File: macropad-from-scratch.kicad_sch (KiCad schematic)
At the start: 23 parts, among them J1 AVR-ISP-6, U1 PRTR5V0U2X, U2 ATmega32U4-A, Y1 Crystal_GND24_Small

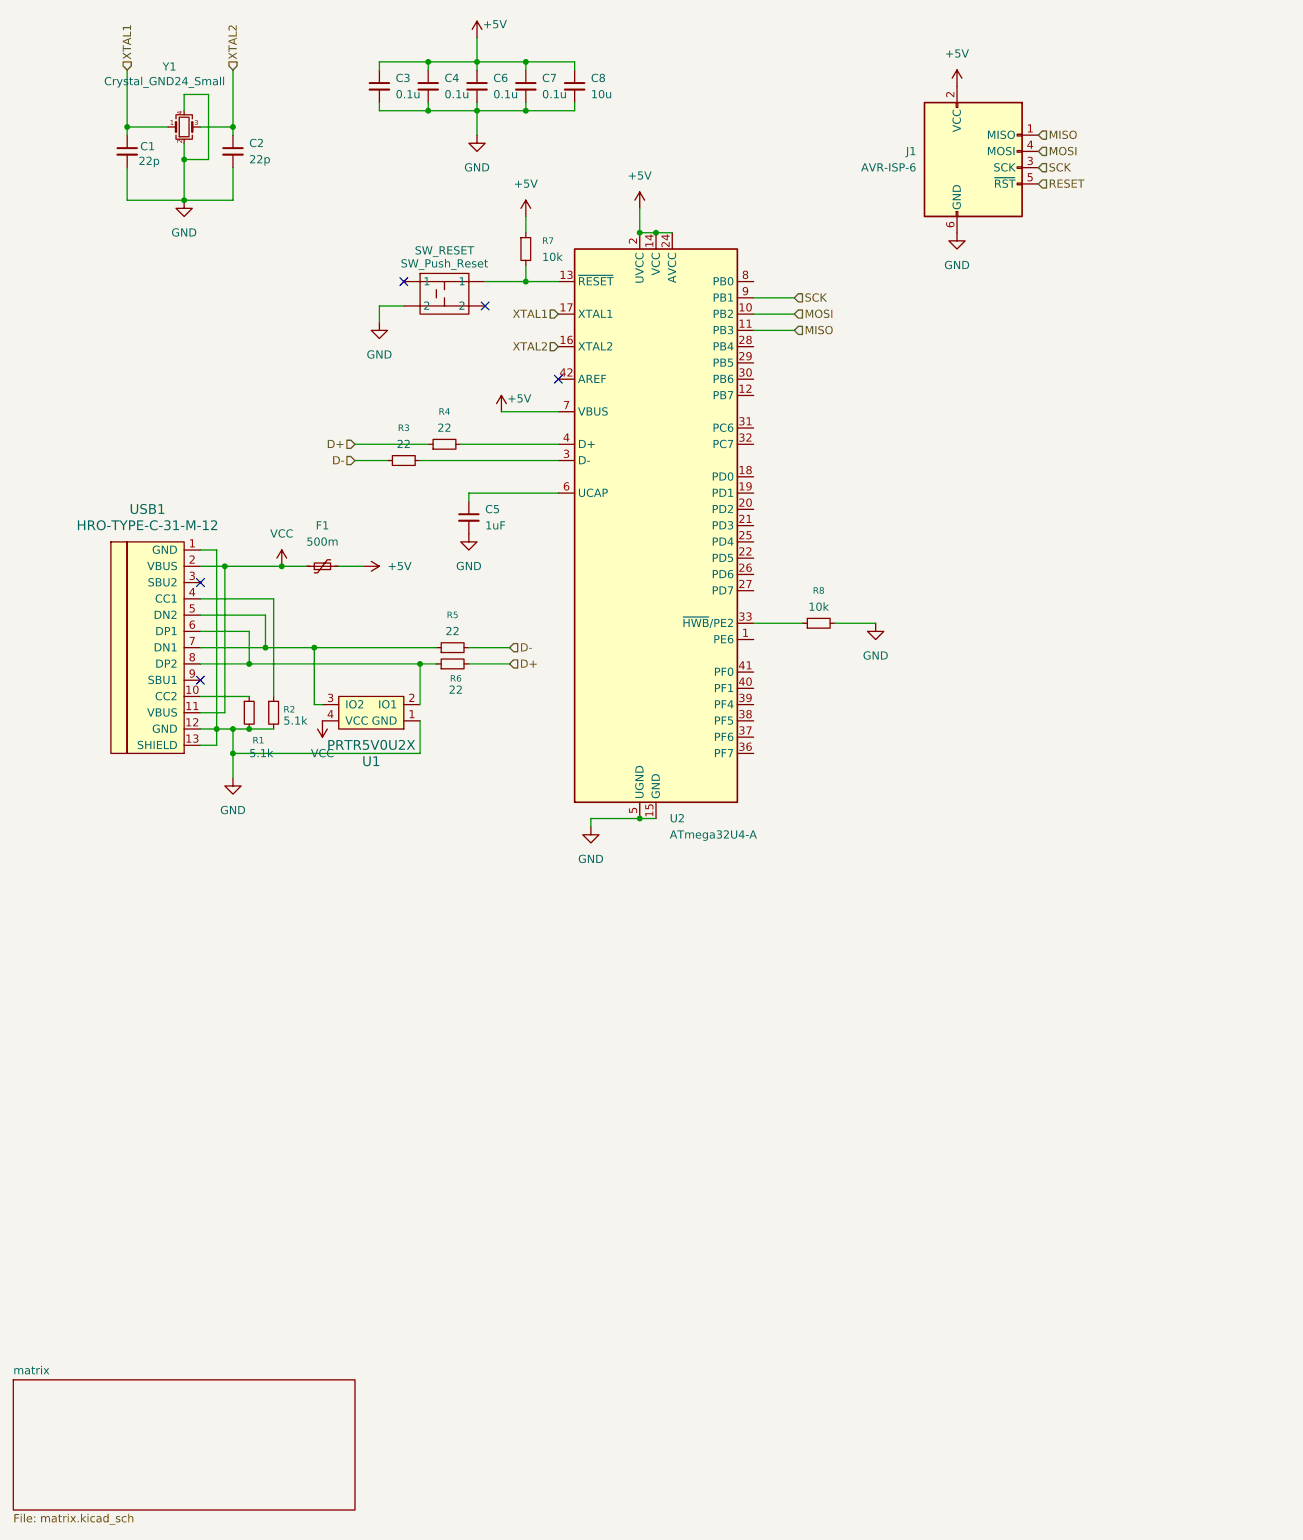
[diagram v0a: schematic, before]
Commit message: completed pcb
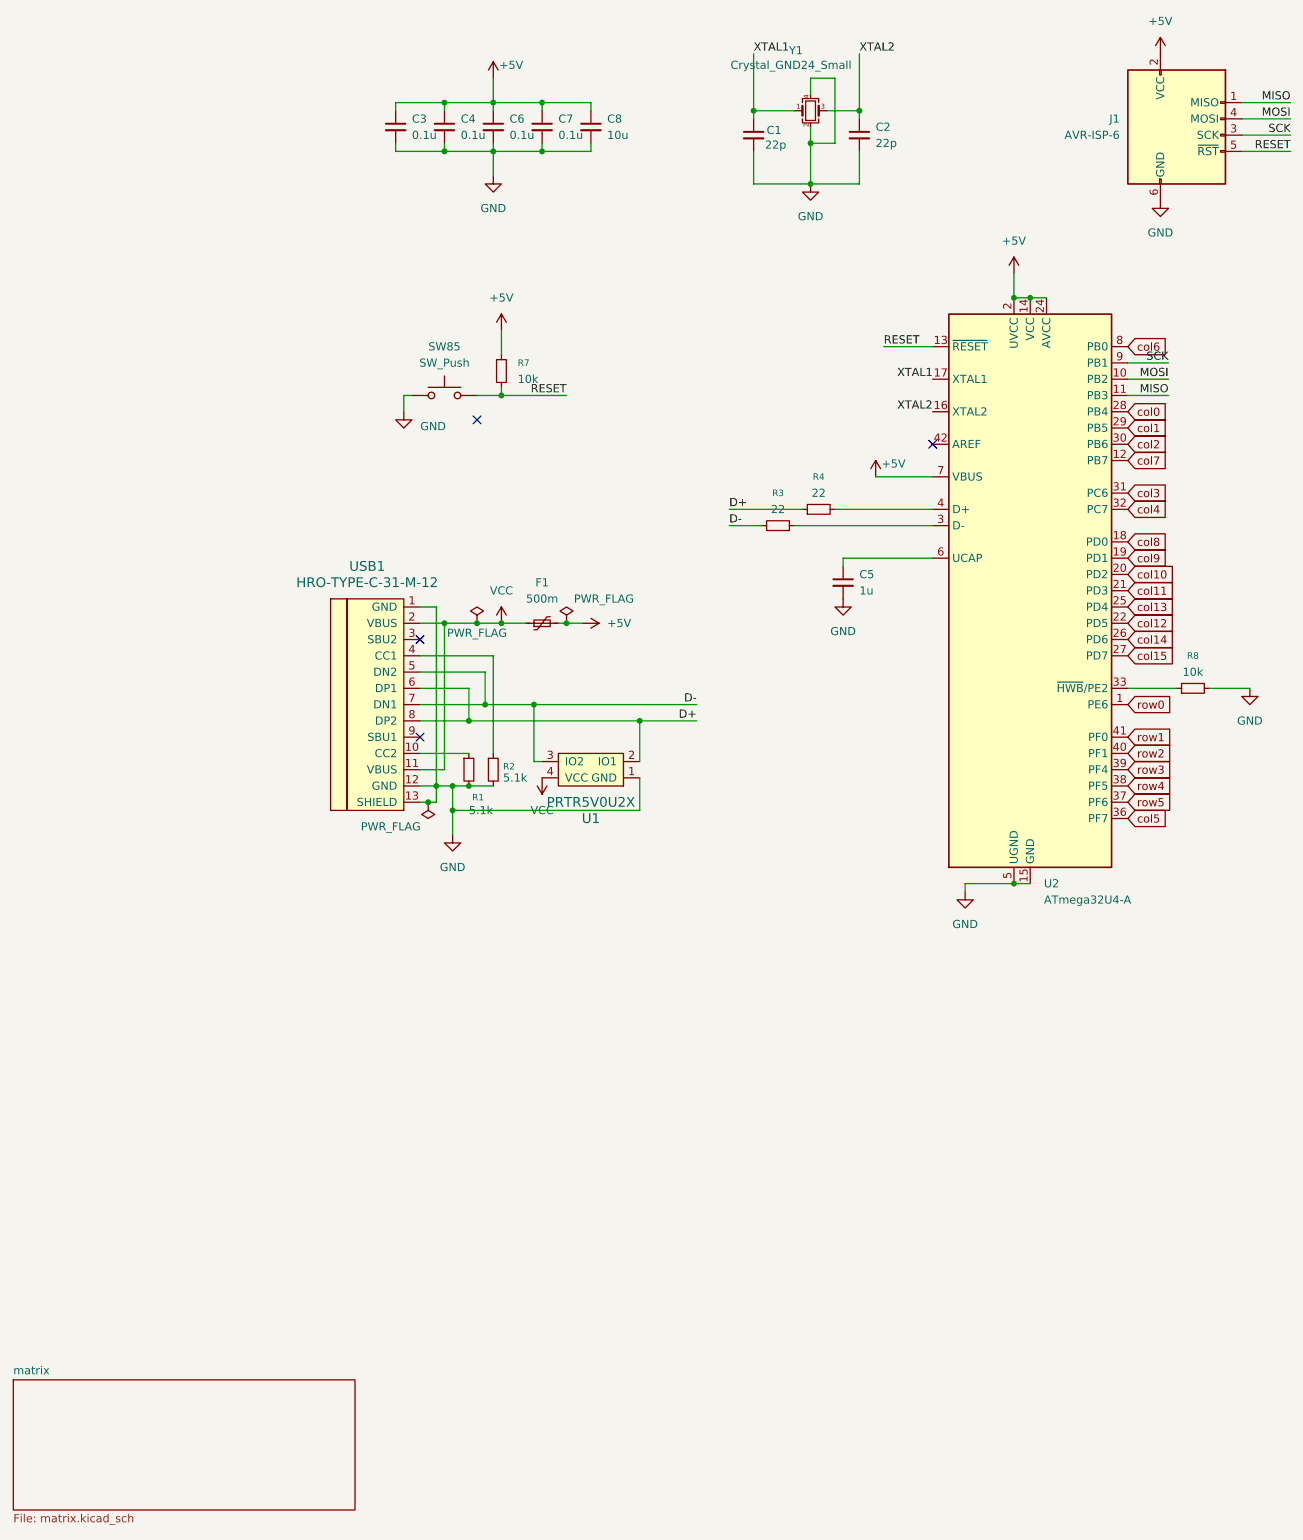
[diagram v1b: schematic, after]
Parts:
- removed R5, R6: 22, symbol Device:R_Small
- removed SW_RESET: SW_Push_Reset, symbol local:SW_PN
- added SW85: SW_Push, Button_Switch_SMD:SW_SPST_SKQG_WithStem, symbol Switch:SW_Push
- C1, C2, C3, C4, C6, C7, C8: footprint (none) -> Capacitor_SMD:C_0805_2012Metric_Pad1.18x1.45mm_HandSolder
- C5: value 1uF -> 1u; footprint (none) -> Capacitor_SMD:C_0805_2012Metric_Pad1.18x1.45mm_HandSolder
- F1: footprint (none) -> Fuse:Fuse_1206_3216Metric_Pad1.42x1.75mm_HandSolder
- J1: footprint (none) -> random-keyboard-parts:Reset_Pretty-Mask
- R1, R2, R3, R4, R7, R8: footprint (none) -> Resistor_SMD:R_0805_2012Metric_Pad1.20x1.40mm_HandSolder
- U1: footprint (none) -> random-keyboard-parts:SOT143B
- USB1: footprint (none) -> Type-C:HRO-TYPE-C-31-M-12-HandSoldering
- Y1: footprint (none) -> Crystal:Crystal_SMD_3225-4Pin_3.2x2.5mm_HandSoldering
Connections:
- net D+: now also U1.2 (IO1), USB1.6 (DP1), USB1.8 (DP2)
- net D-: now also U1.3 (IO2), USB1.5 (DN2), USB1.7 (DN1)
- net GND: now also SW85.1
- net RESET: now also R7.2, U2.13 (~{RESET}), SW85.2
- net row0: now reaches U2.1 (PE6)
- net col7: now reaches U2.12 (PB7)
- net col8: now reaches U2.18 (PD0)
- net col9: now reaches U2.19 (PD1)
- net col10: now reaches U2.20 (PD2)
- net col11: now reaches U2.21 (PD3)
- net col12: now reaches U2.22 (PD5)
- net col13: now reaches U2.25 (PD4)
- net col14: now reaches U2.26 (PD6)
- net col15: now reaches U2.27 (PD7)
- net col0: now reaches U2.28 (PB4)
- net col1: now reaches U2.29 (PB5)
- net col2: now reaches U2.30 (PB6)
- net col3: now reaches U2.31 (PC6)
- net col4: now reaches U2.32 (PC7)
- net col5: now reaches U2.36 (PF7)
- net row5: now reaches U2.37 (PF6)
- net row4: now reaches U2.38 (PF5)
- net row3: now reaches U2.39 (PF4)
- net row2: now reaches U2.40 (PF1)
- net row1: now reaches U2.41 (PF0)
- net col6: now reaches U2.8 (PB0)
- no-connect marks 5 -> 4
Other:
- moved on the sheet: C1, C2, C3, C4, C5, C6, C7, C8, F1, J1, R1, R2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
